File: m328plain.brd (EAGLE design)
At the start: 57.1 x 25.7 mm, 22 parts, among them IC1 7805, J1 PWR, U1 ATMEGA328P_PDIP, Y1 16MHz

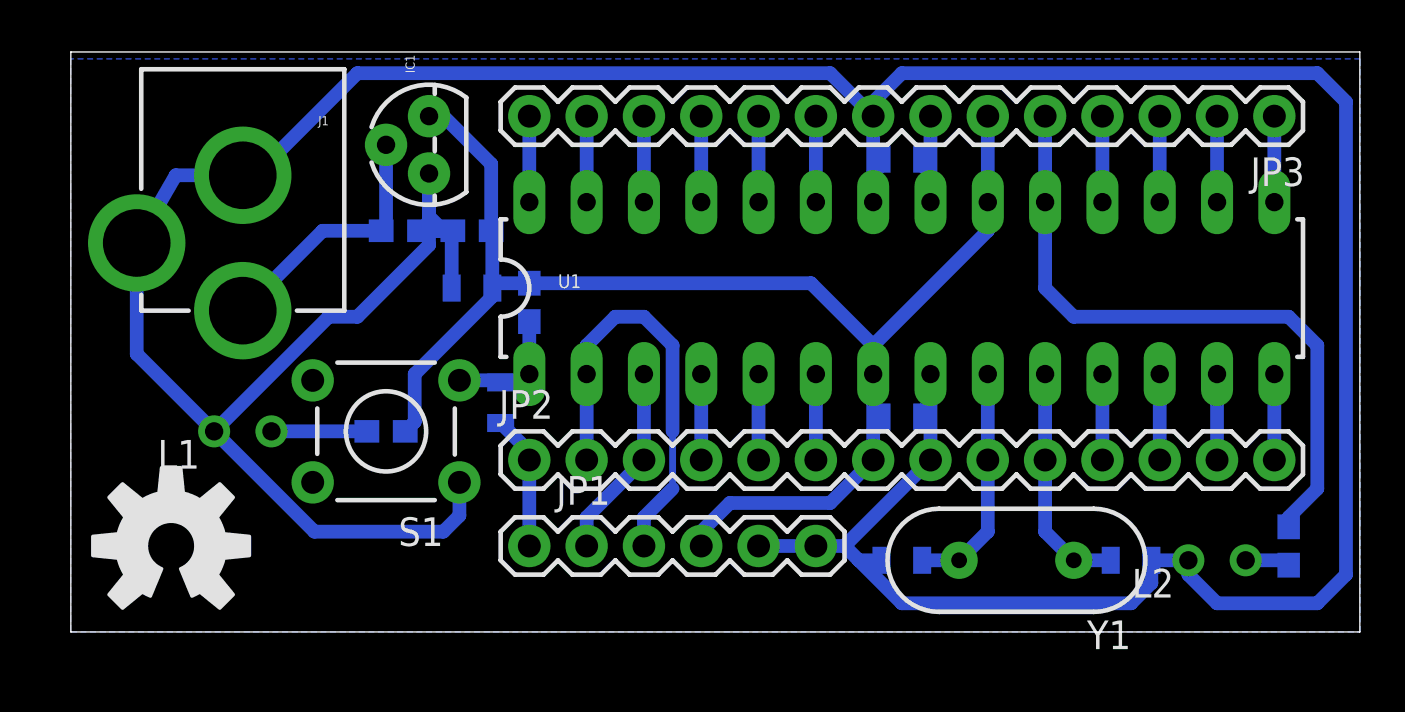
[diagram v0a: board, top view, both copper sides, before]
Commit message: :sparkles: new board layout
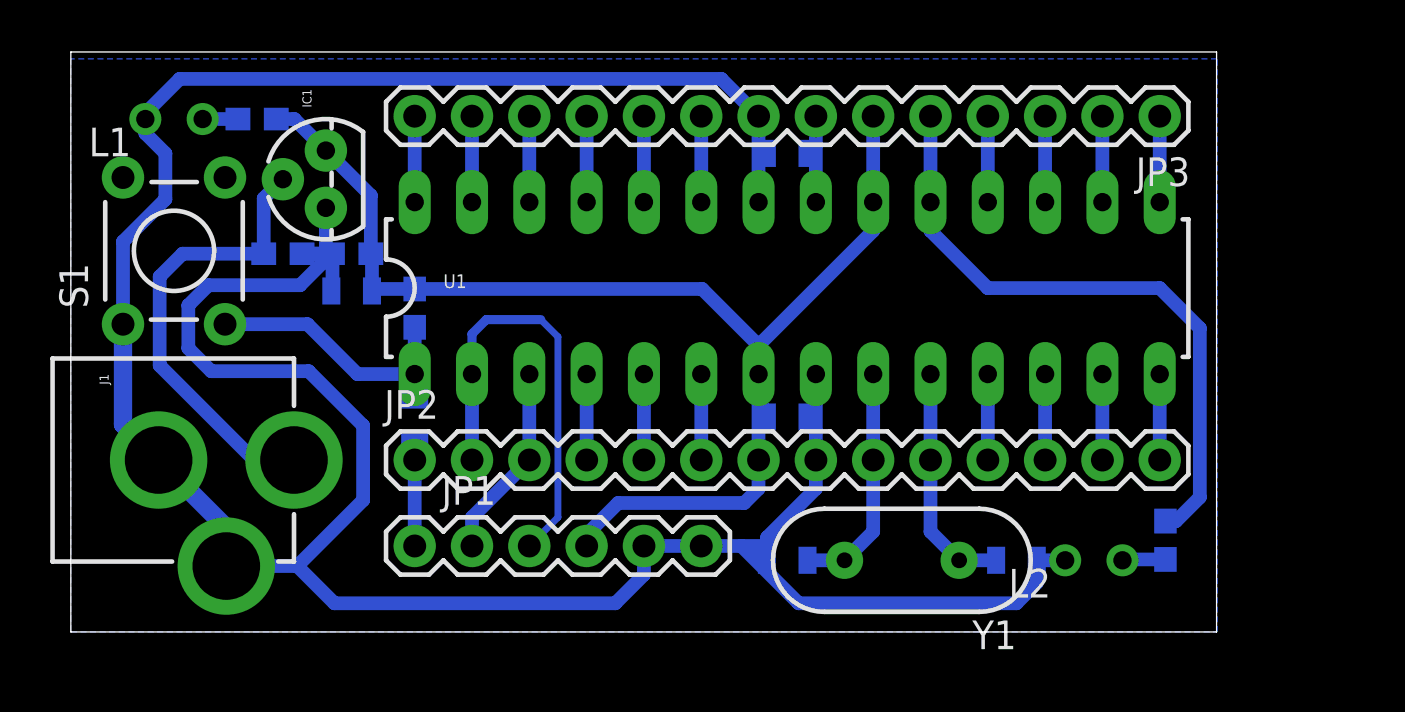
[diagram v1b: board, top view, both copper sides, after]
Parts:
- removed LOGO1: OSHW-LOGOL, SparkFun-Aesthetics:OSHW-LOGO-L
- moved J1 23.3 mm to (-3.81, 6.35), turned to 270 degrees
- moved R3 15.0 mm to (8.26, 21.5)
- moved L1 14.2 mm to (4.57, 21.5)
- moved S1 12.3 mm to (4.57, 15.6), turned to 90 degrees
- moved R2 5.47 mm to (48.5, 2.79)
- moved L2 5.46 mm to (45.3, 1.91)
- moved C7 5.43 mm to (12.4, 15.5)
- moved C5 5.34 mm to (12.4, 13.8)
- moved C6 5.31 mm to (9.40, 15.5)
- moved R1 5.09 mm to (15.2, 13.1)
- moved C4 5.09 mm to (31.8, 19.9)
- moved C1 5.08 mm to (41.9, 1.91)
- moved JP3 5.08 mm to (48.3, 21.6)
- moved JP1 5.08 mm to (15.2, 2.54)
- moved JP2 5.08 mm to (15.2, 6.35)
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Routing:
- net GND: track 175.1 -> 140.9 mm
- net N$9: track 11.5 -> 20.3 mm
- net VCC: track 62.9 -> 56.4 mm
- net N$3: track 6.96 -> 12.5 mm
- net N$10: track 4.23 -> 1.56 mm
- net RST: track 5.98 -> 4.69 mm
- net SCK: track 29.3 -> 28.3 mm
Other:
- board size 57.1 x 25.7 mm -> 50.8 x 25.7 mm
